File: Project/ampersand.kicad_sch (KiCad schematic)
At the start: 19 parts, among them J1 JST SH, U1 STM32F072CBT6

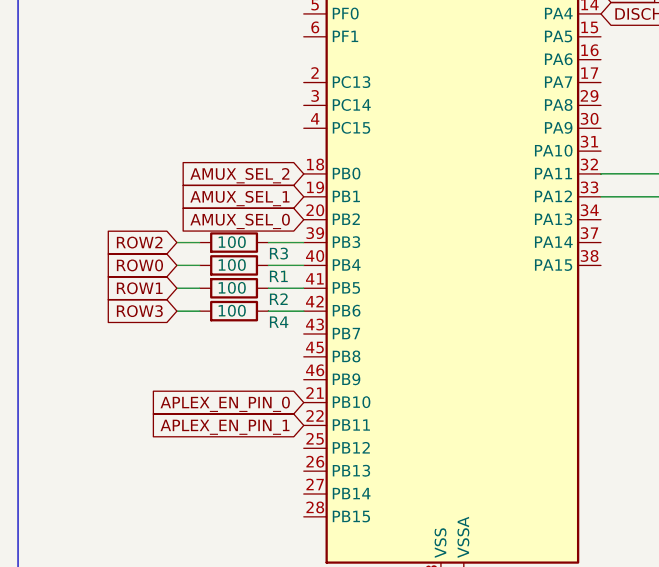
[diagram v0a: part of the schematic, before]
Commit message: clean up
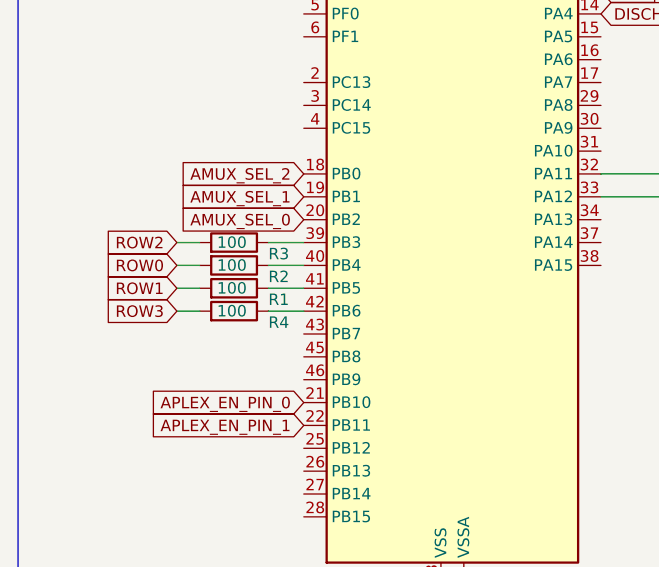
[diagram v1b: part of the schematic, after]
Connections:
- net ROW0: now also R2.2; no longer R1.2
- net ROW1: now also R1.2; no longer R2.2
- net at R1.1: now also U1.41 (PB5); no longer U1.40 (PB4)
- net at R2.1: now also U1.40 (PB4); no longer U1.41 (PB5)
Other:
- moved on the sheet: R1, R2
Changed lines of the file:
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@@
     )
   )
-  (symbol (lib_id "Device:R") (at 38.3592 70.7989 270) (mirror x) (unit 1)
-    (in_bom yes) (on_board yes) (dnp no)
-    (property "Reference" "R1" (at 42.1692 72.0689 90)
-      (effects (font (size 1.27 1.27)) (justify left))
-    )
-    (property "Value" "100" (at 36.4542 70.7989 90)
-      (effects (font (size 1.27 1.27)) (justify left))
-    )
-    (property "Footprint" "Resistor_SMD:R_0402_1005Metric" (at 38.3592 72.5769 90)
-      (effects (font (size 1.27 1.27)) hide)
-    )
-    (property "Datasheet" "~" (at 38.3592 70.7989 0)
-      (effects (font (size 1.27 1.27)) hide)
-    )
-    (property "LCSC" "C25076" (at 38.3592 70.7989 0)
+  (symbol (lib_id "Device:R") (at 38.3592 73.3389 270) (mirror x) (unit 1)
+    (in_bom yes) (on_board yes) (dnp no)
+    (property "Reference" "R1" (at 42.1692 74.6089 90)
+      (effects (font (size 1.27 1.27)) (justify left))
+    )
+    (property "Value" "100" (at 36.4542 73.3389 90)
+      (effects (font (size 1.27 1.27)) (justify left))
+    )
+    (property "Footprint" "Resistor_SMD:R_0402_1005Metric" (at 38.3592 75.1169 90)
+      (effects (font (size 1.27 1.27)) hide)
+    )
+    (property "Datasheet" "~" (at 38.3592 73.3389 0)
+      (effects (font (size 1.27 1.27)) hide)
+    )
+    (property "LCSC" "C25076" (at 38.3592 73.3389 0)
       (effects (font (size 1.27 1.27)) hide)
     )
@@
     )
   )
-  (symbol (lib_id "Device:R") (at 38.3592 73.3389 270) (unit 1)
-    (in_bom yes) (on_board yes) (dnp no)
-    (property "Reference" "R2" (at 42.1692 74.6089 90)
-      (effects (font (size 1.27 1.27)) (justify left))
-    )
-    (property "Value" "100" (at 36.4542 73.3389 90)
-      (effects (font (size 1.27 1.27)) (justify left))
-    )
-    (property "Footprint" "Resistor_SMD:R_0402_1005Metric" (at 38.3592 71.5609 90)
-      (effects (font (size 1.27 1.27)) hide)
-    )
-    (property "Datasheet" "~" (at 38.3592 73.3389 0)
-      (effects (font (size 1.27 1.27)) hide)
-    )
-    (property "LCSC" "C25076" (at 38.3592 73.3389 0)
-      (effects (font (size 1.27 1.27)) hide)
-    )
+  (symbol (lib_id "Device:R") (at 38.3592 70.7989 270) (unit 1)
+    (in_bom yes) (on_board yes) (dnp no)
+    (property "Reference" "R2" (at 42.1692 72.0689 90)
+      (effects (font (size 1.27 1.27)) (justify left))
+    )
+    (property "Value" "100" (at 36.4542 70.7989 90)
+      (effects (font (size 1.27 1.27)) (justify left))
+    )
+    (property "Footprint" "Resistor_SMD:R_0402_1005Metric" (at 38.3592 69.0209 90)
+      (effects (font (size 1.27 1.27)) hide)
+    )
+    (property "Datasheet" "~" (at 38.3592 70.7989 0)
+      (effects (font (size 1.27 1.27)) hide)
+    )
+    (property "LCSC" "C25076" (at 38.3592 70.7989 0)
+      (effects (font (size 1.27 1.27)) hide)
+    )

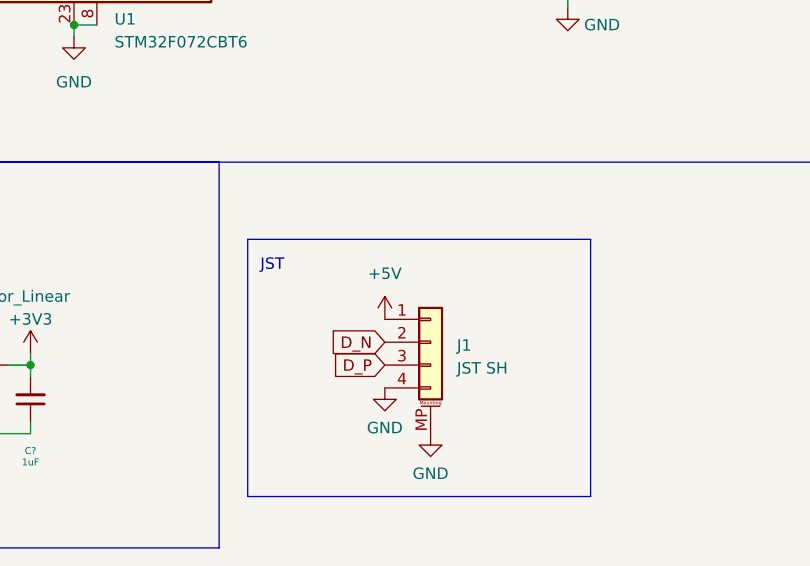
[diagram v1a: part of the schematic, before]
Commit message: plate work
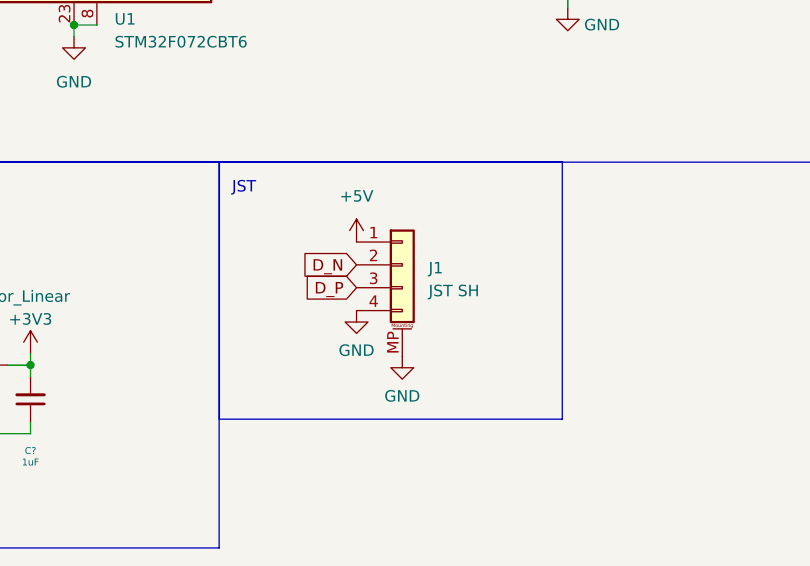
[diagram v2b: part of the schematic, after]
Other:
- moved on the sheet: J1
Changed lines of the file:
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@@
     (stroke (width 0) (type default))
   )
-  (rectangle (start 80.645 130.175) (end 118.745 158.75)
+  (rectangle (start 77.4995 121.5797) (end 115.5995 150.1547)
     (stroke (width 0) (type default))
     (fill (type none))
@@
     (effects (font (size 1.27 1.27)) (justify left bottom))
   )
-  (text "JST" (at 82.042 133.858 0)
+  (text "JST" (at 78.8965 125.2627 0)
     (effects (font (size 1.27 1.27)) (justify left bottom))
   )
@@
     )
   )
-  (global_label "D_N" (shape input) (at 95.885 141.605 180) (fields_autoplaced)
+  (global_label "D_N" (shape input) (at 92.7395 133.0097 180) (fields_autoplaced)
     (effects (font (size 1.27 1.27)) (justify right))
-    (property "Intersheetrefs" "${INTERSHEET_REFS}" (at 89.9038 141.6844 0)
+    (property "Intersheetrefs" "${INTERSHEET_REFS}" (at 86.7583 133.0891 0)
       (effects (font (size 1.27 1.27)) (justify right) hide)
     )
@@
     )
   )
-  (global_label "D_P" (shape input) (at 95.885 144.145 180) (fields_autoplaced)
+  (global_label "D_P" (shape input) (at 92.7395 135.5497 180) (fields_autoplaced)
     (effects (font (size 1.27 1.27)) (justify right))
-    (property "Intersheetrefs" "${INTERSHEET_REFS}" (at 89.4716 144.145 0)
+    (property "Intersheetrefs" "${INTERSHEET_REFS}" (at 86.3261 135.5497 0)
       (effects (font (size 1.27 1.27)) (justify right) hide)
     )
@@
     )
   )
-  (symbol (lib_id "power:+5V") (at 95.885 139.065 0) (unit 1)
+  (symbol (lib_id "power:+5V") (at 92.7395 130.4697 0) (unit 1)
     (in_bom yes) (on_board yes) (dnp no) (fields_autoplaced)
-    (property "Reference" "#PWR0102" (at 95.885 142.875 0)
-      (effects (font (size 1.27 1.27)) hide)
-    )
-    (property "Value" "+5V" (at 95.885 133.985 0)
-      (effects (font (size 1.27 1.27)))
-    )
-    (property "Footprint" "" (at 95.885 139.065 0)
-      (effects (font (size 1.27 1.27)) hide)
-    )
-    (property "Datasheet" "" (at 95.885 139.065 0)
+    (property "Reference" "#PWR0102" (at 92.7395 134.2797 0)
+      (effects (font (size 1.27 1.27)) hide)
+    )
+    (property "Value" "+5V" (at 92.7395 125.3897 0)
+      (effects (font (size 1.27 1.27)))
+    )
+    (property "Footprint" "" (at 92.7395 130.4697 0)
+      (effects (font (size 1.27 1.27)) hide)
+    )
+    (property "Datasheet" "" (at 92.7395 130.4697 0)
       (effects (font (size 1.27 1.27)) hide)
     )
@@
     )
   )
-  (symbol (lib_id "power:GND") (at 100.965 151.765 0) (unit 1)
+  (symbol (lib_id "power:GND") (at 97.8195 143.1697 0) (unit 1)
     (in_bom yes) (on_board yes) (dnp no) (fields_autoplaced)
-    (property "Reference" "#PWR013" (at 100.965 158.115 0)
-      (effects (font (size 1.27 1.27)) hide)
-    )
-    (property "Value" "GND" (at 100.965 156.2084 0)
-      (effects (font (size 1.27 1.27)))
-    )
-    (property "Footprint" "" (at 100.965 151.765 0)
-      (effects (font (size 1.27 1.27)) hide)
-    )
-    (property "Datasheet" "" (at 100.965 151.765 0)
+    (property "Reference" "#PWR013" (at 97.8195 149.5197 0)
+      (effects (font (size 1.27 1.27)) hide)
+    )
+    (property "Value" "GND" (at 97.8195 147.6131 0)
+      (effects (font (size 1.27 1.27)))
+    )
+    (property "Footprint" "" (at 97.8195 143.1697 0)
+      (effects (font (size 1.27 1.27)) hide)
+    )
+    (property "Datasheet" "" (at 97.8195 143.1697 0)
       (effects (font (size 1.27 1.27)) hide)
     )
@@
     )
   )
-  (symbol (lib_id "Connector_Generic_MountingPin:Conn_01x04_MountingPin") (at 100.965 141.605 0) (unit 1)
+  (symbol (lib_id "Connector_Generic_MountingPin:Conn_01x04_MountingPin") (at 97.8195 133.0097 0) (unit 1)
     (in_bom yes) (on_board yes) (dnp no) (fields_autoplaced)
-    (property "Reference" "J1" (at 103.886 141.9605 0)
-      (effects (font (size 1.27 1.27)) (justify left))
-    )
-    (property "Value" "JST SH" (at 103.886 144.5005 0)
-      (effects (font (size 1.27 1.27)) (justify left))
-    )
-    (property "Footprint" "Connector_JST:JST_SH_SM04B-SRSS-TB_1x04-1MP_P1.00mm_Horizontal" (at 100.965 141.605 0)
-      (effects (font (size 1.27 1.27)) hide)
-    )
-    (property "Datasheet" "~" (at 100.965 141.605 0)
+    (property "Reference" "J1" (at 100.7405 133.3652 0)
+      (effects (font (size 1.27 1.27)) (justify left))
+    )
+    (property "Value" "JST SH" (at 100.7405 135.9052 0)
+      (effects (font (size 1.27 1.27)) (justify left))
+    )
+    (property "Footprint" "Connector_JST:JST_SH_SM04B-SRSS-TB_1x04-1MP_P1.00mm_Horizontal" (at 97.8195 133.0097 0)
+      (effects (font (size 1.27 1.27)) hide)
+    )
+    (property "Datasheet" "~" (at 97.8195 133.0097 0)
       (effects (font (size 1.27 1.27)) hide)
     )
@@
     )
   )
-  (symbol (lib_id "power:GND") (at 95.885 146.685 0) (unit 1)
+  (symbol (lib_id "power:GND") (at 92.7395 138.0897 0) (unit 1)
     (in_bom yes) (on_board yes) (dnp no) (fields_autoplaced)
-    (property "Reference" "#PWR011" (at 95.885 153.035 0)
-      (effects (font (size 1.27 1.27)) hide)
-    )
-    (property "Value" "GND" (at 95.885 151.1284 0)
-      (effects (font (size 1.27 1.27)))
-    )
-    (property "Footprint" "" (at 95.885 146.685 0)
-      (effects (font (size 1.27 1.27)) hide)
-    )
-    (property "Datasheet" "" (at 95.885 146.685 0)
-      (effects (font (size 1.27 1.27)) hide)
-    )
+    (property "Reference" "#PWR011" (at 92.7395 144.4397 0)
+      (effects (font (size 1.27 1.27)) hide)
+    )
+    (property "Value" "GND" (at 92.7395 142.5331 0)
+      (effects (font (size 1.27 1.27)))
+    )
+    (property "Footprint" "" (at 92.7395 138.0897 0)
+      (effects (font (size 1.27 1.27)) hide)
+    )
+    (property "Datasheet" "" (at 92.7395 138.0897 0)
+      (effects (font (size 1.27 1.27)) hide)
+    )
